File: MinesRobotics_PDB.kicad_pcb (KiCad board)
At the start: 2 copper layers, 109.2 x 127 mm, 37 parts, among them J1 Conn_01x02, J10 Conn_01x02, J11 Conn_01x02, J12 Conn_01x02, J13 Conn_01x02, J14 Conn_02x03_Odd_Even, J15 Conn_01x07, J2 Conn_01x02, J3 Conn_01x02, J4 Conn_01x02, J5 Conn_01x02, J6 Conn_01x02, J7 Conn_01x02, J8 Conn_01x02, J9 Conn_01x02, K1 DIPxx-1Axx-12x, Q1 Q_NMOS_GSD, SW1 SW_Push, U1 R-78E5.0-1.0, U2 ATtiny85-20SU

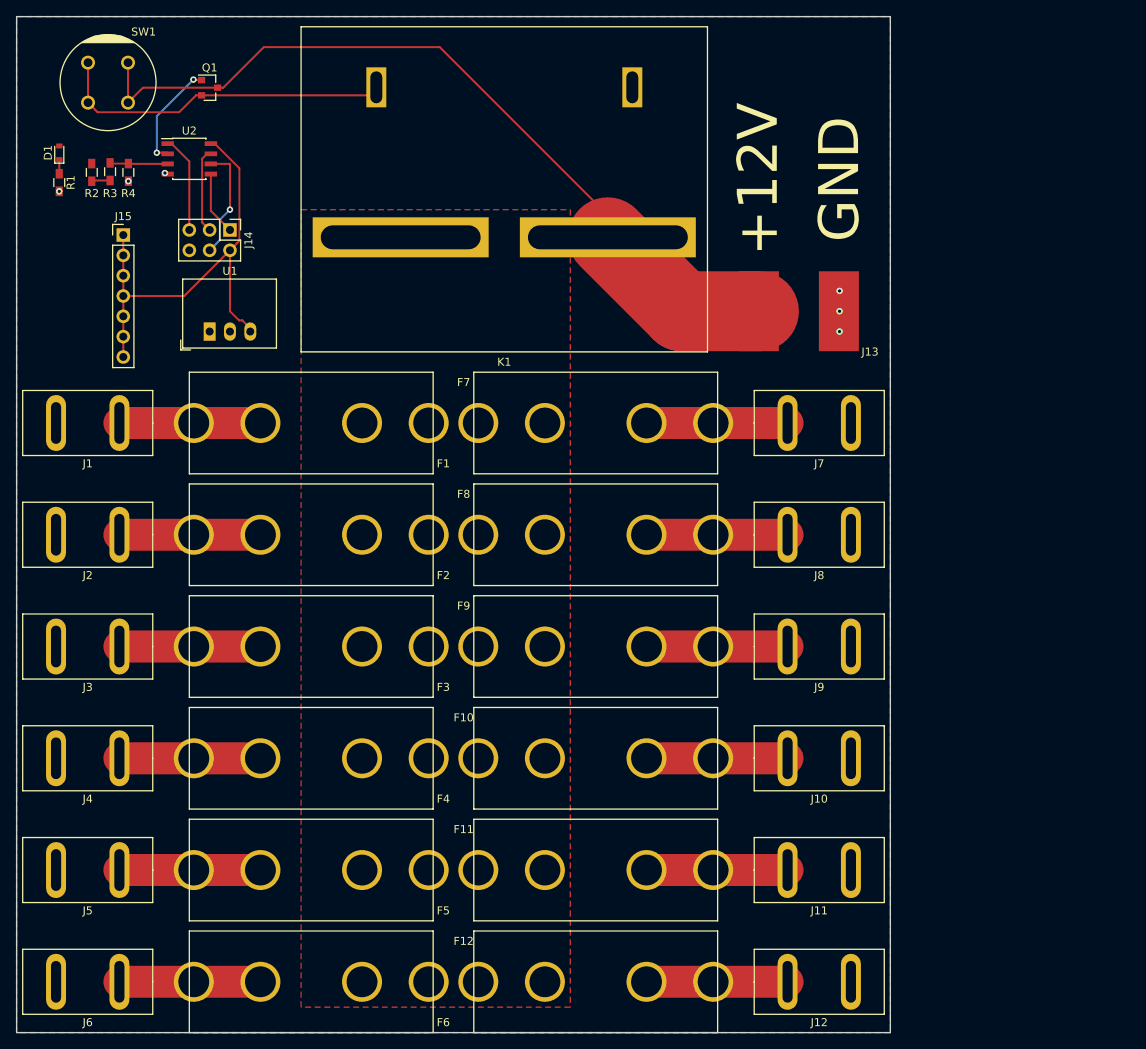
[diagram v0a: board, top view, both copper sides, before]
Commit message: Initial commit
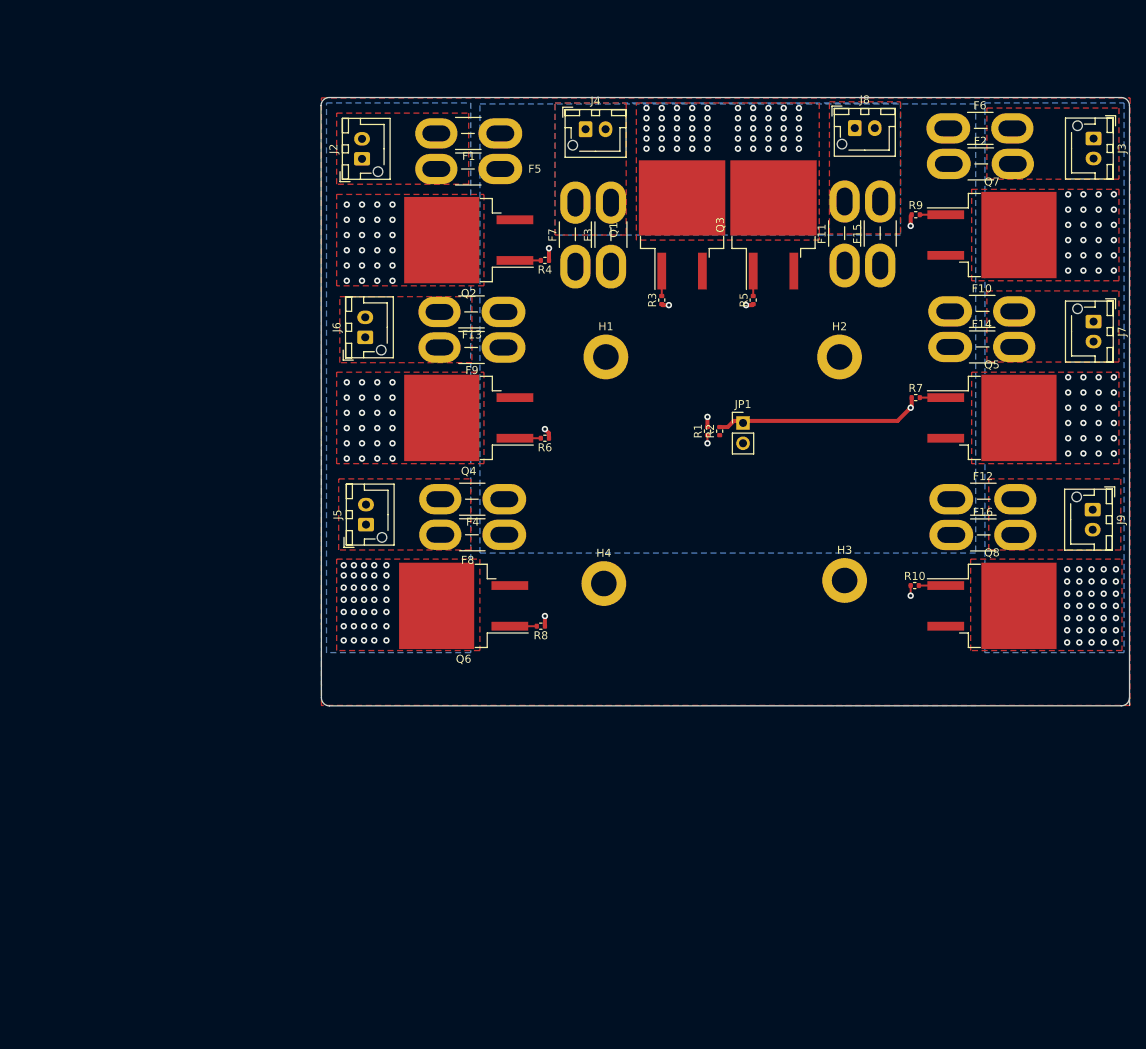
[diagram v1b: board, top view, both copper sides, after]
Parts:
- removed D1: LED, Diodes_SMD:D_0603
- removed J1, J10, J11, J12: Conn_01x02, Kicad_Fprint:PowerPole_45A_Vert
- removed J13: Conn_01x02, Kicad_Fprint:12AWG_SolderPad
- removed J14: Conn_02x03_Odd_Even, Connector_PinHeader_2.54mm:PinHeader_2x03_P2.54mm_Vertical
- removed J15: Conn_01x07, Connector_PinHeader_2.54mm:PinHeader_1x07_P2.54mm_Vertical
- removed K1: DIPxx-1Axx-12x, Kicad_Fprint:HE1AN-W-DC24V-Y7
- removed SW1: SW_Push, Kicad_Fprint:KS-01Q-01
- removed U1: R-78E5.0-1.0, Converter_DCDC:Converter_DCDC_RECOM_R-78E-0.5_THT
- removed U2: ATtiny85-20SU, Housings_SOIC:SOIC-8_3.9x4.9mm_Pitch1.27mm
- added F13: Fuse, Fuse:Fuse_Blade_Mini_directSolder, F.Cu at (104.0, 77.6)
- added F14: Fuse, Fuse:Fuse_Blade_Mini_directSolder, F.Cu at (159.9, 81.9)
- added F15: Fuse, Fuse:Fuse_Blade_Mini_directSolder, F.Cu at (151.1, 71.8)
- added F16: Fuse, Fuse:Fuse_Blade_Mini_directSolder, F.Cu at (160.0, 105.4)
- added H1: MountingHole_Pad, MountingHole:MountingHole_3.2mm_M3_DIN965_Pad, F.Cu at (116.8, 83.2)
- added H2: MountingHole_Pad, MountingHole:MountingHole_3.2mm_M3_DIN965_Pad, F.Cu at (146.1, 83.2)
- added H3: MountingHole_Pad, MountingHole:MountingHole_3.2mm_M3_DIN965_Pad, F.Cu at (146.7, 111.1)
- added H4: MountingHole_Pad, MountingHole:MountingHole_3.2mm_M3_DIN965_Pad, F.Cu at (116.6, 111.5)
- added JP1: Jumper_2_Open, Connector_PinHeader_2.54mm:PinHeader_1x02_P2.54mm_Vertical, F.Cu at (134.0, 91.4)
- added Q2: IRFS3607TRLPBF, Package_TO_SOT_SMD:TO-263-2, F.Cu at (99.7, 68.6)
- added Q3: IRFS3607TRLPBF, Package_TO_SOT_SMD:TO-263-2, F.Cu at (137.8, 66.7)
- added Q4: IRFS3607TRLPBF, Package_TO_SOT_SMD:TO-263-2, F.Cu at (99.7, 90.8)
- added Q5: IRFS3607TRLPBF, Package_TO_SOT_SMD:TO-263-2, F.Cu at (165.1, 90.8)
- added Q6: IRFS3607TRLPBF, Package_TO_SOT_SMD:TO-263-2, F.Cu at (99.1, 114.3)
- added Q7: IRFS3607TRLPBF, Package_TO_SOT_SMD:TO-263-2, F.Cu at (165.1, 67.9)
- added Q8: IRFS3607TRLPBF, Package_TO_SOT_SMD:TO-263-2, F.Cu at (165.1, 114.3)
- added R10: 10, Resistor_SMD:R_0402_1005Metric, F.Cu at (155.4, 111.8)
- added R5: 10, Resistor_SMD:R_0402_1005Metric, F.Cu at (135.3, 76.1)
- added R6: 10, Resistor_SMD:R_0402_1005Metric, F.Cu at (109.2, 93.3)
- added R7: 10, Resistor_SMD:R_0402_1005Metric, F.Cu at (155.6, 88.3)
- added R8: 10, Resistor_SMD:R_0402_1005Metric, F.Cu at (108.7, 116.8)
- added R9: 10, Resistor_SMD:R_0402_1005Metric, F.Cu at (155.6, 65.4)
- F1, F10, F11, F12, F2, F3, F4, F5, F6, F7, F8, F9: value 60A -> Fuse; footprint Kicad_Fprint:3555-2 Maxi FuseHolder -> Fuse:Fuse_Blade_Mini_directSolder
- J2, J3, J4, J5, J6, J7, J8, J9: value Conn_01x02 -> Conn_01x02_Female; footprint Kicad_Fprint:PowerPole_45A_Vert -> Connector_JST:JST_XH_B2B-XH-AM_1x02_P2.50mm_Vertical
- Q1: value Q_NMOS_GSD -> IRFS3607TRLPBF; footprint TO_SOT_Packages_SMD:SOT-23 -> Package_TO_SOT_SMD:TO-263-2
- R1: value 1k -> 21k; footprint Resistors_SMD:R_0603_HandSoldering -> Resistor_SMD:R_0402_1005Metric
- R2: value 1k -> 15k; footprint Resistors_SMD:R_0603_HandSoldering -> Resistor_SMD:R_0402_1005Metric
- R3, R4: value 1k -> 10; footprint Resistors_SMD:R_0603_HandSoldering -> Resistor_SMD:R_0402_1005Metric
- moved J3 140.9 mm to (177.8, 55.9)
- moved F6 133.1 mm to (159.6, 54.6)
- moved J4 100.3 mm to (114.3, 54.7), turned to 0 degrees
- moved F2 92.2 mm to (159.7, 59.1)
- moved F5 90.8 mm to (103.6, 59.7), turned to 180 degrees
- moved J6 87.7 mm to (86.8, 80.7), turned to 90 degrees
- moved R1 86.8 mm to (129.5, 92.5), turned to 90 degrees
- moved R2 84.9 mm to (131.1, 92.5), turned to 90 degrees
- moved F11 81.7 mm to (146.7, 71.8), turned to 90 degrees
- moved F12 74.9 mm to (160.0, 101.0), turned to 0 degrees
- moved F10 71.3 mm to (159.9, 77.5), turned to 0 degrees
- moved R3 70.8 mm to (123.8, 76.1)
- moved Q1 61.5 mm to (126.4, 66.7), turned to 90 degrees
- moved F3 60.5 mm to (117.5, 71.9), turned to 90 degrees
- moved J2 58.2 mm to (86.4, 58.4), turned to 90 degrees
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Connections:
- F1 pad 1: Net-(F1-Pad1) -> +24V
- F1 pad 2: +12V -> /Fuses/DRIVE_MOTOR_LEFT_FRONT
- F10 pad 1: Net-(F10-Pad1) -> +24V
- F10 pad 2: +12V -> /Fuses/DRIVE_MOTOR_RIGHT_REAR
- F11 pad 1: Net-(F11-Pad1) -> +24V
- F11 pad 2: +12V -> /Fuses/AUX2_MOTORS1
- F12 pad 1: Net-(F12-Pad1) -> +24V
- F12 pad 2: +12V -> /Fuses/AUX2_MOTORS2
- F2 pad 1: Net-(F2-Pad1) -> +24V
- F2 pad 2: +12V -> /Fuses/DRIVE_MOTOR_RIGHT_FRONT
- F3 pad 1: Net-(F3-Pad1) -> +24V
- F3 pad 2: +12V -> /Fuses/AUX1_MOTORS1
- F4 pad 1: Net-(F4-Pad1) -> +24V
- F4 pad 2: +12V -> /Fuses/AUX1_MOTORS2
- F5 pad 1: Net-(F5-Pad1) -> +24V
- F5 pad 2: +12V -> /Fuses/DRIVE_MOTOR_LEFT_FRONT
- F6 pad 1: Net-(F6-Pad1) -> +24V
- F6 pad 2: +12V -> /Fuses/DRIVE_MOTOR_RIGHT_FRONT
- F7 pad 1: Net-(F7-Pad1) -> +24V
- F7 pad 2: +12V -> /Fuses/AUX1_MOTORS1
- F8 pad 1: Net-(F8-Pad1) -> +24V
- F8 pad 2: +12V -> /Fuses/AUX1_MOTORS2
- F9 pad 1: Net-(F9-Pad1) -> +24V
- F9 pad 2: +12V -> /Fuses/DRIVE_MOTOR_LEFT_REAR
- J2 pad 1: Net-(F2-Pad1) -> /Fuses/DRIVE_MOTOR_LEFT_FRONT
- J2 pad 2: GND -> /Battery Power Distribution/DRIVE_MOTORS_LEFT
- J3 pad 1: Net-(F3-Pad1) -> /Fuses/DRIVE_MOTOR_RIGHT_FRONT
- J3 pad 2: GND -> /Battery Power Distribution/DRIVE_MORTORS_RIGHT
- J4 pad 1: Net-(F4-Pad1) -> /Fuses/AUX1_MOTORS1
- J4 pad 2: GND -> /Battery Power Distribution/AUX_MOTORS
- J5 pad 1: Net-(F5-Pad1) -> /Fuses/AUX1_MOTORS2
- J5 pad 2: GND -> /Battery Power Distribution/DRIVE_MOTORS_LEFT
- J6 pad 1: Net-(F6-Pad1) -> /Fuses/DRIVE_MOTOR_LEFT_REAR
- J6 pad 2: GND -> /Battery Power Distribution/DRIVE_MOTORS_LEFT
- J7 pad 1: Net-(F7-Pad1) -> /Fuses/DRIVE_MOTOR_RIGHT_REAR
- J7 pad 2: GND -> /Battery Power Distribution/DRIVE_MORTORS_RIGHT
- J8 pad 1: Net-(F8-Pad1) -> /Fuses/AUX2_MOTORS1
- J8 pad 2: GND -> /Battery Power Distribution/AUX_MOTORS
- J9 pad 1: Net-(F9-Pad1) -> /Fuses/AUX2_MOTORS2
- J9 pad 2: GND -> /Battery Power Distribution/DRIVE_MORTORS_RIGHT
- Q1 pad 1: /Battery_Control -> Net-(Q1-Pad1)
- Q1 pad 2: Net-(K1-Pad6) -> /Battery Power Distribution/AUX_MOTORS
- Q1 pad 3: /Vbat -> GND
- R1 pad 1: Net-(D1-Pad1) -> +24V
- R1 pad 2: GND -> /Battery Power Distribution/GATE_DRIVE
- R2 pad 1: +12V -> GND
- R2 pad 2: Net-(R2-Pad2) -> /Battery Power Distribution/GATE_DRIVE
- R3 pad 1: Net-(R2-Pad2) -> /Battery Power Distribution/GATE_DRIVE
- R3 pad 2: Net-(R3-Pad2) -> Net-(Q1-Pad1)
- R4 pad 1: Net-(R3-Pad2) -> /Battery Power Distribution/GATE_DRIVE
- R4 pad 2: GND -> Net-(Q2-Pad1)
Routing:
- net /Battery Power Distribution/GATE_DRIVE: track 0.00 -> 193.2 mm, vias 0 -> 9
- net /Vbat: track 102.0 -> 0.00 mm
- net +5V: track 58.0 -> 0.00 mm
- net Net-(K1-Pad6): track 42.8 -> 0.00 mm
- net Net-(F9-Pad1): track 17.6 -> 0.00 mm
- net Net-(F8-Pad1): track 17.6 -> 0.00 mm
- net Net-(F7-Pad1): track 17.6 -> 0.00 mm
- net Net-(F12-Pad1): track 17.6 -> 0.00 mm
- net Net-(F11-Pad1): track 17.6 -> 0.00 mm
- net Net-(F10-Pad1): track 17.6 -> 0.00 mm
- net Net-(F6-Pad1): track 17.6 -> 0.00 mm
- net Net-(F5-Pad1): track 17.6 -> 0.00 mm
- net Net-(F4-Pad1): track 17.6 -> 0.00 mm
- net Net-(F3-Pad1): track 17.6 -> 0.00 mm
- net Net-(F2-Pad1): track 17.6 -> 0.00 mm
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- added copper zone on B.Cu, net +24V
- added copper zone on B.Cu, net /Battery Power Distribution/AUX_MOTORS
- added copper zone on F.Cu, net /Battery Power Distribution/AUX_MOTORS
- added copper zone on B.Cu, net /Battery Power Distribution/DRIVE_MORTORS_RIGHT
- added copper zone on F.Cu, net /Battery Power Distribution/DRIVE_MORTORS_RIGHT
- added copper zone on B.Cu, net /Battery Power Distribution/DRIVE_MOTORS_LEFT
- added copper zone on F.Cu, net /Battery Power Distribution/DRIVE_MOTORS_LEFT
- added copper zone on F.Cu, net /Fuses/AUX1_MOTORS1
- added copper zone on F.Cu, net /Fuses/AUX1_MOTORS2
- added copper zone on F.Cu, net /Fuses/AUX2_MOTORS1
- added copper zone on F.Cu, net /Fuses/AUX2_MOTORS2
- added copper zone on F.Cu, net /Fuses/DRIVE_MOTOR_LEFT_FRONT
- added copper zone on F.Cu, net /Fuses/DRIVE_MOTOR_LEFT_REAR
- added copper zone on F.Cu, net /Fuses/DRIVE_MOTOR_RIGHT_FRONT
- added copper zone on F.Cu, net /Fuses/DRIVE_MOTOR_RIGHT_REAR
- added copper zone on F.Cu, net GND
- removed copper zone on F.Cu, net +12V
- removed copper zone on B.Cu, net GND
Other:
- board size 109.2 x 127 mm -> 101.1 x 76 mm
- copper layers 2 -> 4
- net class Default removed
- board text removed: "+12V"
- board text removed: "GND"
